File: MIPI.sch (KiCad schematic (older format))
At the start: 42 parts, among them J8 ARJP11A-MASA-B-A-EMU2, J9 MIPI, U1 AllWinner-S3(FBGA-234), Y2 32.768kHz, Y3 24MHz

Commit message: update
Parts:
- removed J8: ARJP11A-MASA-B-A-EMU2, Connector_RJ:RJ45_Abracon_ARJP11A-MA_Horizontal, symbol Connector:RJ45_Abracon_ARJP11A-MASA-B-A-EMU2
- added J?: HR961160C, otter:HR961160C, symbol otter:HR961160C
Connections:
- net labels removed: POE_POWER_N, POE_POWER_P
- wire segments 125 -> 137
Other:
- moved on the sheet: C100, C101, C102, C103, C104, J9, R90, R91, R92, R93, R94

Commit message: update
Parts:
- removed J?: HR961160C, otter:HR961160C, symbol otter:HR961160C
- added J?: 49F-1201GYD2NL, otter:49F-1201GYDXNL, symbol otter:49F-1201GYD2NL
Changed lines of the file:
@@
 Wire Wire Line
 	1900 2300 2700 2300
-$Comp
-L otter:HR961160C J?
-U 1 1 60385DAB
-P 7550 2300
-F 0 "J?" H 7020 2346 50  0000 R CNN
-F 1 "HR961160C" H 7020 2255 50  0000 R CNN
-F 2 "otter:HR961160C" H 7150 1750 50  0001 C CNN
-F 3 "https://productfinder.pulseeng.com/doc_type/WEB301/doc_num/JXD6-0001NL/doc_part/JXD6-0001NL.pdf" H 7135 2065 50  0001 L TNN
-	1    7550 2300
-	1    0    0    -1
-$EndComp
-$Comp
-L S3-OLinuXino_Rev_A:GND #PWR?
-U 1 1 603969A5
-P 8200 2750
-AR Path="/5D8A1FAC/603969A5" Ref="#PWR?"  Part="1"
-AR Path="/603969A5" Ref="#PWR?"  Part="1"
-AR Path="/620E795B/603969A5" Ref="#PWR?"  Part="1"
-F 0 "#PWR?" H 8200 2500 50  0001 C CNN
-F 1 "GND" H 8200 2600 50  0000 C CNN
-F 2 "" H 8200 2750 60  0000 C CNN
-F 3 "" H 8200 2750 60  0000 C CNN
-	1    8200 2750
-	-1   0    0    -1
-$EndComp
 Wire Wire Line
 	8200 2100 8250 2100
@@
 Wire Wire Line
 	9350 2500 9350 2550
+$Comp
+L otter:49F-1201GYD2NL J?
+U 1 1 60475CA8
+P 7550 2300
+F 0 "J?" H 7020 2346 50  0000 R CNN
+F 1 "49F-1201GYD2NL" H 7020 2255 50  0000 R CNN
+F 2 "otter:49F-1201GYDXNL" H 7150 1750 50  0001 C CNN
+F 3 "https://productfinder.pulseeng.com/doc_type/WEB301/doc_num/JXD6-0001NL/doc_part/JXD6-0001NL.pdf" H 7135 2065 50  0001 L TNN
+	1    7550 2300
+	1    0    0    -1
+$EndComp
 $EndSCHEMATC

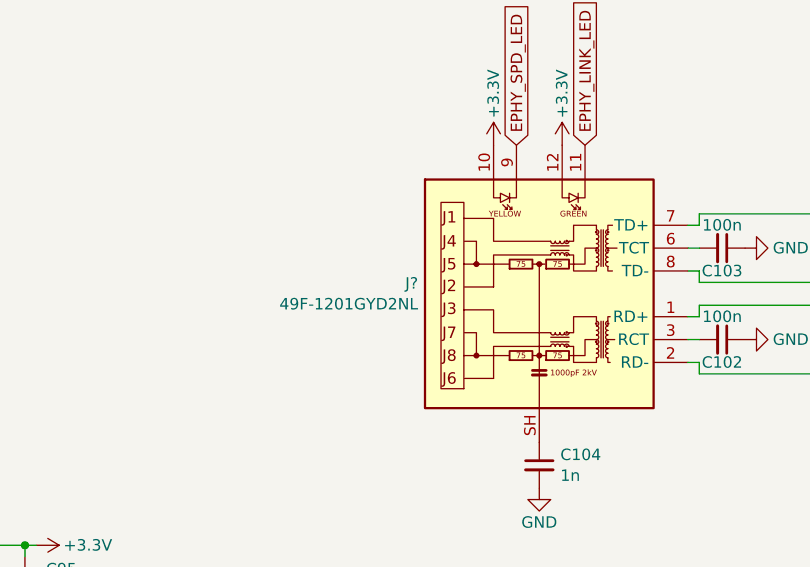
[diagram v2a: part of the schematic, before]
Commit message: update
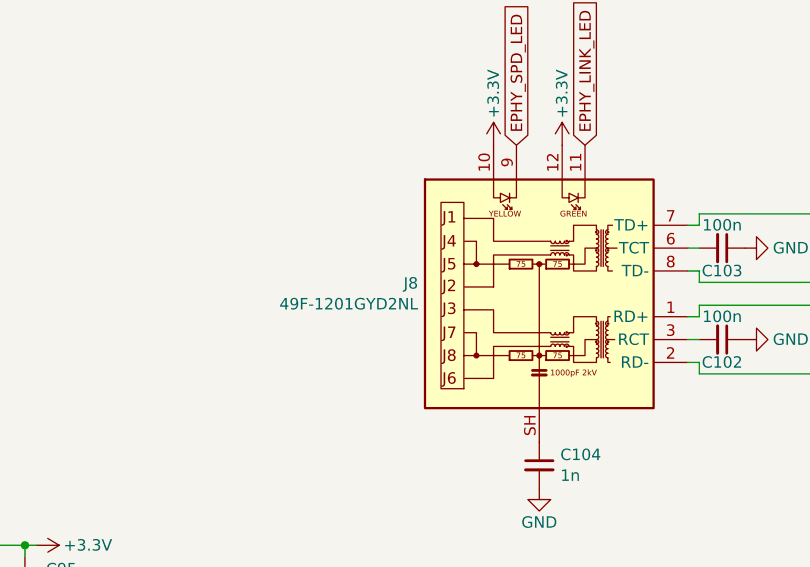
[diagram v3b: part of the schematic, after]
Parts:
- gave numbers to parts that had none: 1
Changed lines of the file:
@@
 	9350 2500 9350 2550
 $Comp
-L otter:49F-1201GYD2NL J?
+L otter:49F-1201GYD2NL J8
 U 1 1 60475CA8
 P 7550 2300
-F 0 "J?" H 7020 2346 50  0000 R CNN
+F 0 "J8" H 7020 2346 50  0000 R CNN
 F 1 "49F-1201GYD2NL" H 7020 2255 50  0000 R CNN
 F 2 "otter:49F-1201GYDXNL" H 7150 1750 50  0001 C CNN

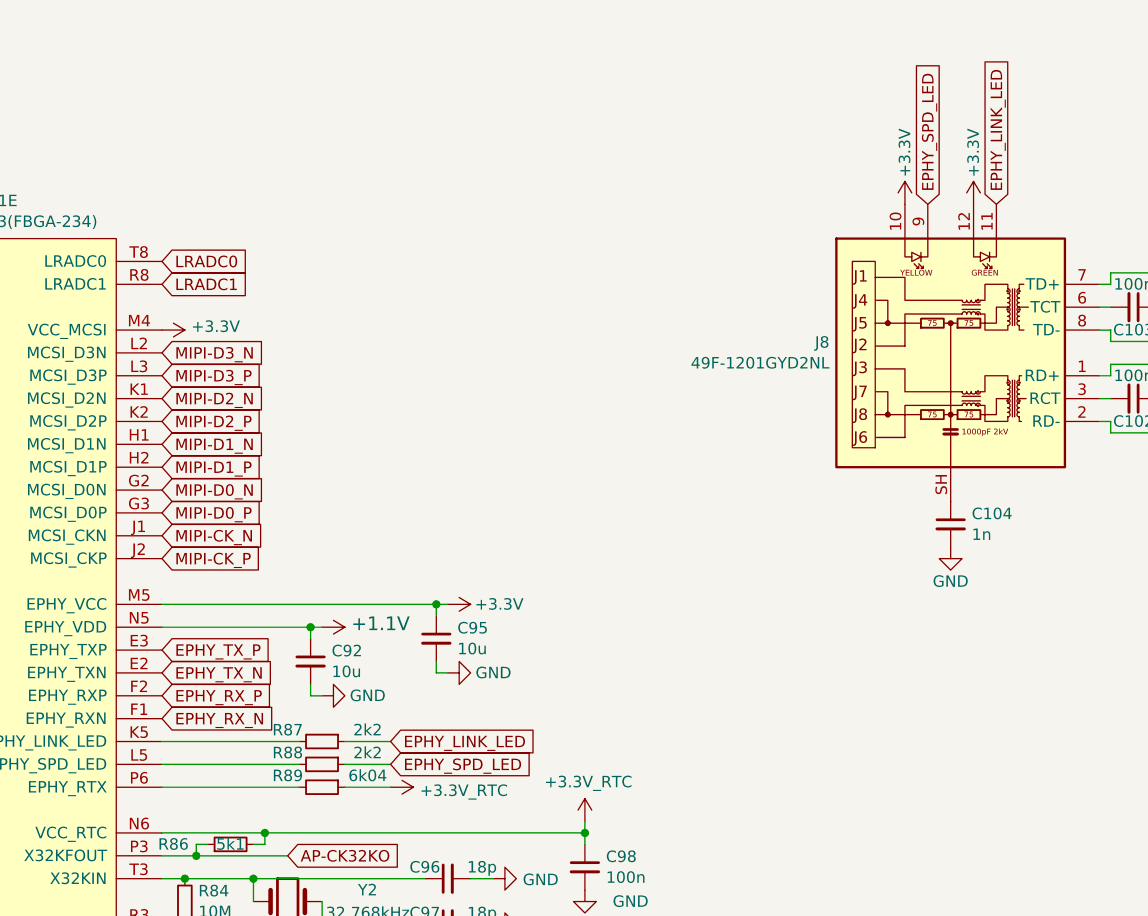
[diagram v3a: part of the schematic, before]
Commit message: update
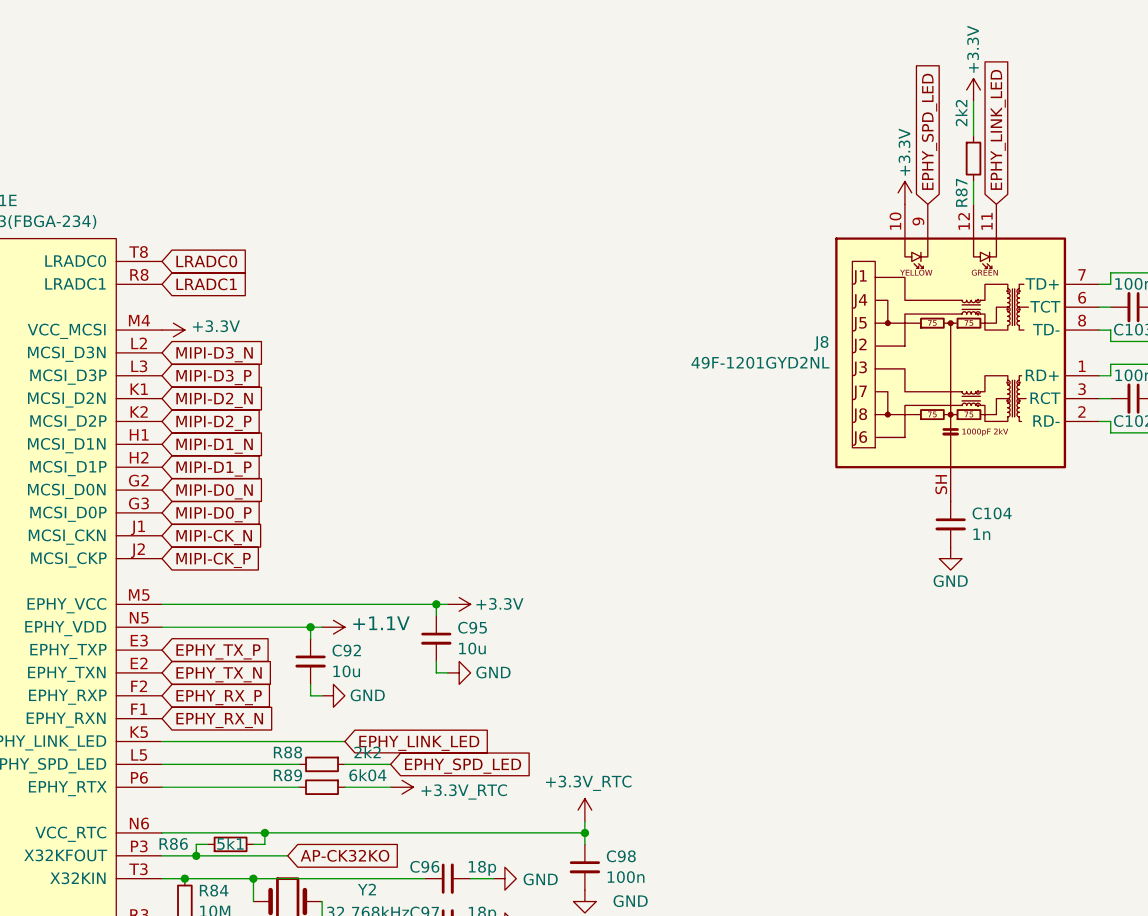
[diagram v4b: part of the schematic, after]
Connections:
- net +3V3: now also R87.1; no longer J8.12
- net EPHY_LINK_LED: now also U1.K5 (EPHY_LINK_LED); no longer R87.1
- net at R87.2: now also J8.12; no longer U1.K5 (EPHY_LINK_LED)
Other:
- moved on the sheet: R87
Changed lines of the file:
@@
 L Device:R_Small R?
 U 1 1 6851960A
-P 4800 4000
+P 7650 1450
 AR Path="/6851960A" Ref="R?"  Part="1"
 AR Path="/620E795B/6851960A" Ref="R87"  Part="1"
-F 0 "R87" V 4750 3850 50  0000 C CNN
-F 1 "2k2" V 4750 4200 50  0000 C CNN
-F 2 "otter:C_0402" H 4800 4000 50  0001 C CNN
-F 3 "~" H 4800 4000 50  0001 C CNN
-	1    4800 4000
-	0    1    1    0
+F 0 "R87" V 7600 1300 50  0000 C CNN
+F 1 "2k2" V 7600 1650 50  0000 C CNN
+F 2 "otter:C_0402" H 7650 1450 50  0001 C CNN
+F 3 "~" H 7650 1450 50  0001 C CNN
+	1    7650 1450
+	1    0    0    -1
 $EndComp
 $Comp
@@
 	0    1    1    0
 $EndComp
-Text GLabel 5100 4000 2    50   Input ~ 0
+Text GLabel 4900 4000 2    50   Input ~ 0
 EPHY_LINK_LED
 Text GLabel 5100 4100 2    50   Input ~ 0
@@
 L S3-OLinuXino_Rev_A:+3.3V #PWR?
 U 1 1 68ABBB53
-P 7650 1650
+P 7650 1200
 AR Path="/5D8A1FAC/68ABBB53" Ref="#PWR?"  Part="1"
 AR Path="/68ABBB53" Ref="#PWR?"  Part="1"
 AR Path="/620E795B/68ABBB53" Ref="#PWR0279"  Part="1"
-F 0 "#PWR0279" H 7650 1500 50  0001 C CNN
-F 1 "+3.3V" V 7650 1875 50  0000 C CNN
-F 2 "" H 7650 1650 60  0000 C CNN
-F 3 "" H 7650 1650 60  0000 C CNN
-	1    7650 1650
+F 0 "#PWR0279" H 7650 1050 50  0001 C CNN
+F 1 "+3.3V" V 7650 1425 50  0000 C CNN
+F 2 "" H 7650 1200 60  0000 C CNN
+F 3 "" H 7650 1200 60  0000 C CNN
+	1    7650 1200
 	-1   0    0    -1
 $EndComp
@@
 $EndComp
 Wire Wire Line
-	4100 4000 4700 4000
-Wire Wire Line
 	4100 4100 4700 4100
 Wire Wire Line
 	4100 4200 4700 4200
-Wire Wire Line
-	4900 4000 5100 4000
 Wire Wire Line
 	4900 4100 5100 4100
@@
 	1    0    0    -1
 $EndComp
+Wire Wire Line
+	4100 4000 4900 4000
+Wire Wire Line
+	7650 1200 7650 1350
+Wire Wire Line
+	7650 1550 7650 1650
 $EndSCHEMATC

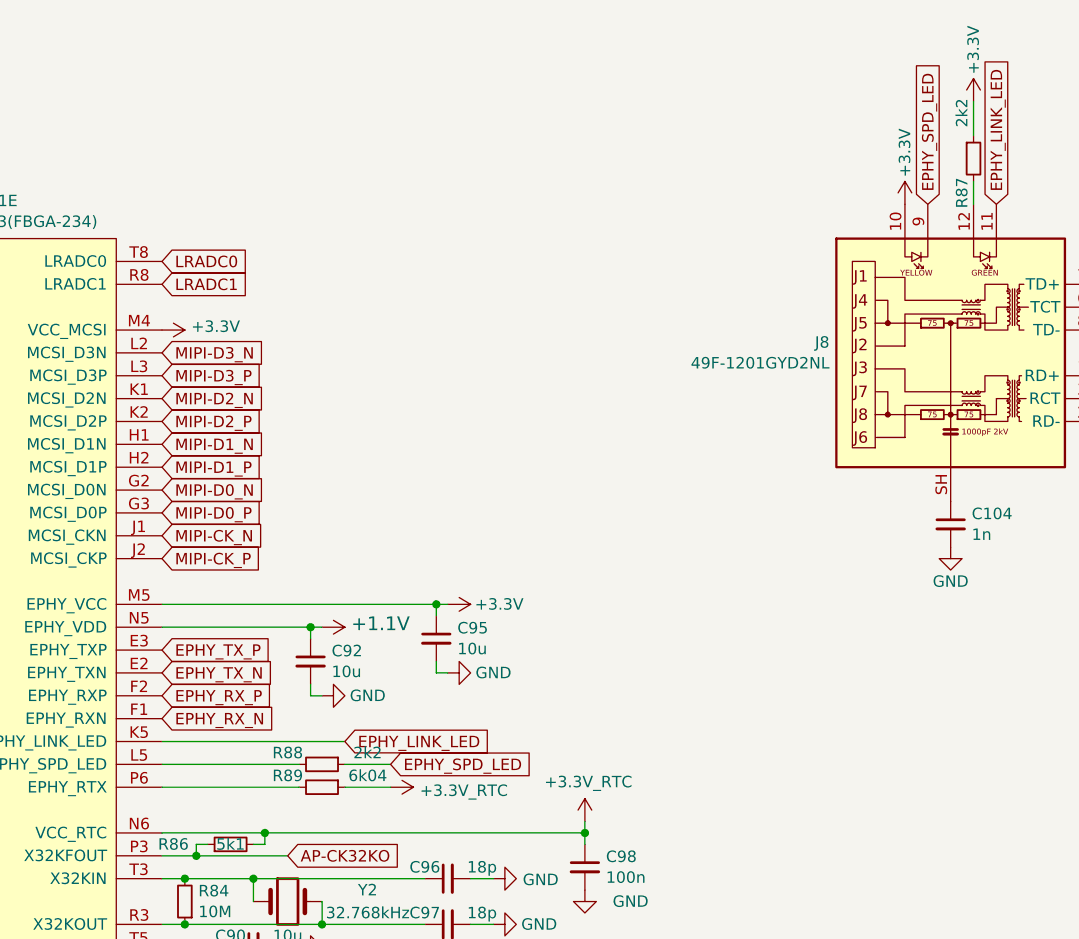
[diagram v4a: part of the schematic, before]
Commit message: update
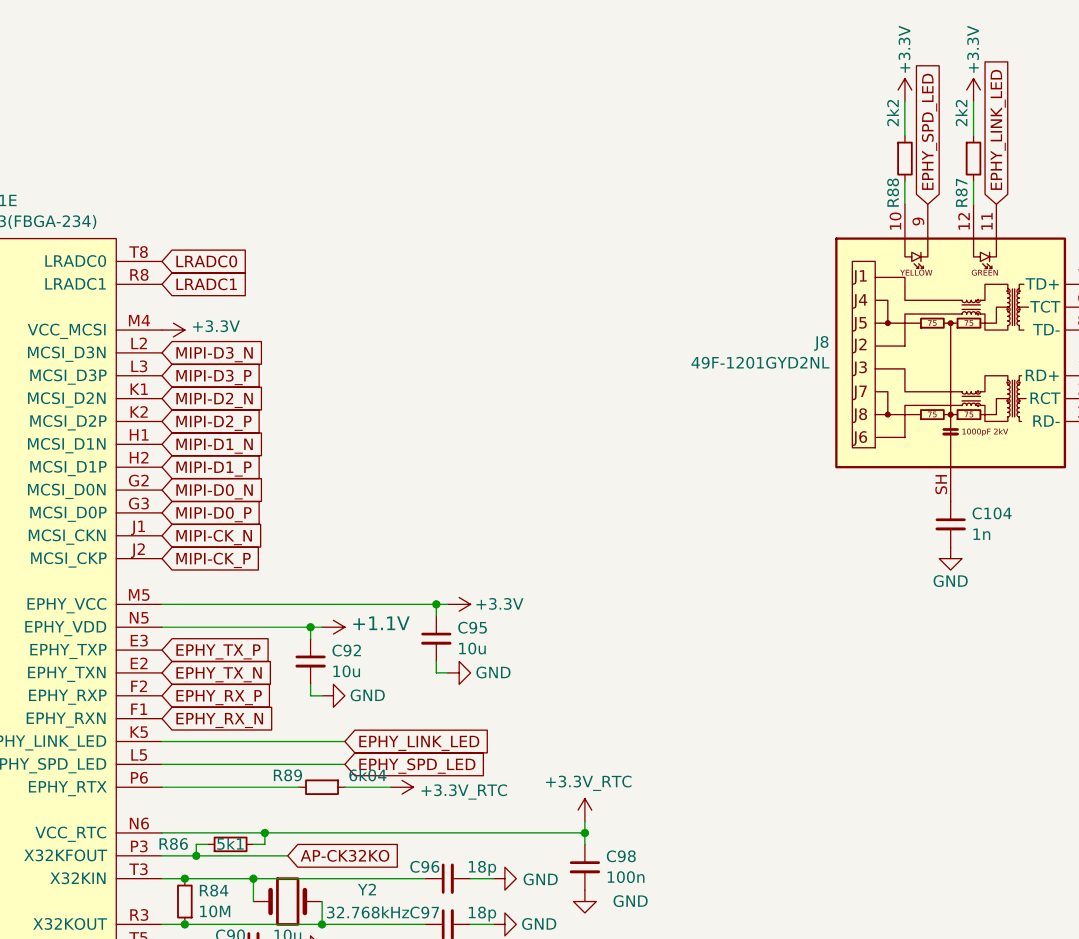
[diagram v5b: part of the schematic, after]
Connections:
- net +3V3: now also R88.1; no longer J8.10
- net EPHY_SPD_LED: now also U1.L5 (EPHY_SPD_LED); no longer R88.1
- net at R88.2: now also J8.10; no longer U1.L5 (EPHY_SPD_LED)
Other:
- moved on the sheet: R88
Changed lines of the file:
@@
 L Device:R_Small R?
 U 1 1 685269CF
-P 4800 4100
+P 7350 1450
 AR Path="/685269CF" Ref="R?"  Part="1"
 AR Path="/620E795B/685269CF" Ref="R88"  Part="1"
-F 0 "R88" V 4750 3950 50  0000 C CNN
-F 1 "2k2" V 4750 4300 50  0000 C CNN
-F 2 "otter:C_0402" H 4800 4100 50  0001 C CNN
-F 3 "~" H 4800 4100 50  0001 C CNN
-	1    4800 4100
-	0    1    1    0
+F 0 "R88" V 7300 1300 50  0000 C CNN
+F 1 "2k2" V 7300 1650 50  0000 C CNN
+F 2 "otter:C_0402" H 7350 1450 50  0001 C CNN
+F 3 "~" H 7350 1450 50  0001 C CNN
+	1    7350 1450
+	1    0    0    -1
 $EndComp
 $Comp
@@
 Text GLabel 4900 4000 2    50   Input ~ 0
 EPHY_LINK_LED
-Text GLabel 5100 4100 2    50   Input ~ 0
+Text GLabel 4900 4100 2    50   Input ~ 0
 EPHY_SPD_LED
 $Comp
@@
 L S3-OLinuXino_Rev_A:+3.3V #PWR?
 U 1 1 68AC8602
-P 7350 1650
+P 7350 1200
 AR Path="/5D8A1FAC/68AC8602" Ref="#PWR?"  Part="1"
 AR Path="/68AC8602" Ref="#PWR?"  Part="1"
 AR Path="/620E795B/68AC8602" Ref="#PWR0280"  Part="1"
-F 0 "#PWR0280" H 7350 1500 50  0001 C CNN
-F 1 "+3.3V" V 7350 1875 50  0000 C CNN
-F 2 "" H 7350 1650 60  0000 C CNN
-F 3 "" H 7350 1650 60  0000 C CNN
-	1    7350 1650
+F 0 "#PWR0280" H 7350 1050 50  0001 C CNN
+F 1 "+3.3V" V 7350 1425 50  0000 C CNN
+F 2 "" H 7350 1200 60  0000 C CNN
+F 3 "" H 7350 1200 60  0000 C CNN
+	1    7350 1200
 	-1   0    0    -1
 $EndComp
@@
 $EndComp
 Wire Wire Line
-	4100 4100 4700 4100
-Wire Wire Line
 	4100 4200 4700 4200
-Wire Wire Line
-	4900 4100 5100 4100
 Wire Wire Line
 	4900 4200 5100 4200
@@
 Wire Wire Line
 	7650 1550 7650 1650
+Wire Wire Line
+	4100 4100 4900 4100
+Wire Wire Line
+	7350 1550 7350 1650
+Wire Wire Line
+	7350 1350 7350 1200
 $EndSCHEMATC

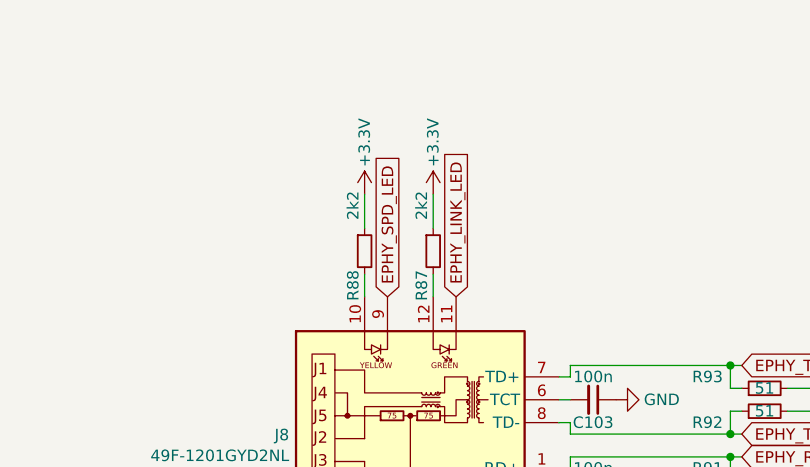
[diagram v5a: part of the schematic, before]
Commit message: update
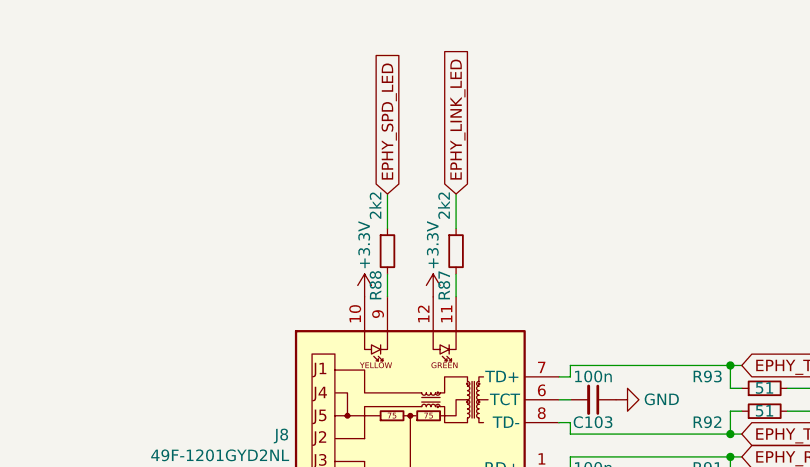
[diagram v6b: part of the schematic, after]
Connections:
- net +3V3: now also J8.10, J8.12; no longer R87.1, R88.1
- net EPHY_LINK_LED: now also R87.1; no longer J8.11
- net EPHY_SPD_LED: now also R88.1; no longer J8.9
- net at R88.2: now also J8.9; no longer J8.10
- net at R87.2: now also J8.11; no longer J8.12
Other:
- moved on the sheet: R87, R88
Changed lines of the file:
@@
 L Device:R_Small R?
 U 1 1 6851960A
-P 7650 1450
+P 7750 1450
 AR Path="/6851960A" Ref="R?"  Part="1"
 AR Path="/620E795B/6851960A" Ref="R87"  Part="1"
-F 0 "R87" V 7600 1300 50  0000 C CNN
-F 1 "2k2" V 7600 1650 50  0000 C CNN
-F 2 "otter:C_0402" H 7650 1450 50  0001 C CNN
-F 3 "~" H 7650 1450 50  0001 C CNN
-	1    7650 1450
+F 0 "R87" V 7700 1300 50  0000 C CNN
+F 1 "2k2" V 7700 1650 50  0000 C CNN
+F 2 "otter:C_0402" H 7750 1450 50  0001 C CNN
+F 3 "~" H 7750 1450 50  0001 C CNN
+	1    7750 1450
 	1    0    0    -1
 $EndComp
@@
 L Device:R_Small R?
 U 1 1 685269CF
-P 7350 1450
+P 7450 1450
 AR Path="/685269CF" Ref="R?"  Part="1"
 AR Path="/620E795B/685269CF" Ref="R88"  Part="1"
-F 0 "R88" V 7300 1300 50  0000 C CNN
-F 1 "2k2" V 7300 1650 50  0000 C CNN
-F 2 "otter:C_0402" H 7350 1450 50  0001 C CNN
-F 3 "~" H 7350 1450 50  0001 C CNN
-	1    7350 1450
+F 0 "R88" V 7400 1300 50  0000 C CNN
+F 1 "2k2" V 7400 1650 50  0000 C CNN
+F 2 "otter:C_0402" H 7450 1450 50  0001 C CNN
+F 3 "~" H 7450 1450 50  0001 C CNN
+	1    7450 1450
 	1    0    0    -1
 $EndComp
@@
 Text GLabel 9000 2650 2    50   Input ~ 0
 EPHY_RX_N
-Text GLabel 7750 1650 1    50   Input ~ 0
+Text GLabel 7750 1200 1    50   Input ~ 0
 EPHY_LINK_LED
-Text GLabel 7450 1650 1    50   Input ~ 0
+Text GLabel 7450 1200 1    50   Input ~ 0
 EPHY_SPD_LED
 $Comp
 L S3-OLinuXino_Rev_A:+3.3V #PWR?
 U 1 1 68ABBB53
-P 7650 1200
+P 7650 1650
 AR Path="/5D8A1FAC/68ABBB53" Ref="#PWR?"  Part="1"
 AR Path="/68ABBB53" Ref="#PWR?"  Part="1"
 AR Path="/620E795B/68ABBB53" Ref="#PWR0279"  Part="1"
-F 0 "#PWR0279" H 7650 1050 50  0001 C CNN
-F 1 "+3.3V" V 7650 1425 50  0000 C CNN
-F 2 "" H 7650 1200 60  0000 C CNN
-F 3 "" H 7650 1200 60  0000 C CNN
-	1    7650 1200
+F 0 "#PWR0279" H 7650 1500 50  0001 C CNN
+F 1 "+3.3V" V 7650 1875 50  0000 C CNN
+F 2 "" H 7650 1650 60  0000 C CNN
+F 3 "" H 7650 1650 60  0000 C CNN
+	1    7650 1650
 	-1   0    0    -1
 $EndComp
@@
 L S3-OLinuXino_Rev_A:+3.3V #PWR?
 U 1 1 68AC8602
-P 7350 1200
+P 7350 1650
 AR Path="/5D8A1FAC/68AC8602" Ref="#PWR?"  Part="1"
 AR Path="/68AC8602" Ref="#PWR?"  Part="1"
 AR Path="/620E795B/68AC8602" Ref="#PWR0280"  Part="1"
-F 0 "#PWR0280" H 7350 1050 50  0001 C CNN
-F 1 "+3.3V" V 7350 1425 50  0000 C CNN
-F 2 "" H 7350 1200 60  0000 C CNN
-F 3 "" H 7350 1200 60  0000 C CNN
-	1    7350 1200
+F 0 "#PWR0280" H 7350 1500 50  0001 C CNN
+F 1 "+3.3V" V 7350 1875 50  0000 C CNN
+F 2 "" H 7350 1650 60  0000 C CNN
+F 3 "" H 7350 1650 60  0000 C CNN
+	1    7350 1650
 	-1   0    0    -1
 $EndComp
@@
 	4100 4000 4900 4000
 Wire Wire Line
-	7650 1200 7650 1350
-Wire Wire Line
-	7650 1550 7650 1650
+	7750 1200 7750 1350
+Wire Wire Line
+	7750 1550 7750 1650
 Wire Wire Line
 	4100 4100 4900 4100
 Wire Wire Line
-	7350 1550 7350 1650
-Wire Wire Line
-	7350 1350 7350 1200
+	7450 1550 7450 1650
+Wire Wire Line
+	7450 1350 7450 1200
 $EndSCHEMATC
